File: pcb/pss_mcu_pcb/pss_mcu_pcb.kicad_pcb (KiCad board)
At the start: 4 copper layers, 30.1 x 47.4 mm, 50 parts, among them J1 STM32_Prog, J2 UART_Prog, J3 Conn_01x18, J4 Conn_01x18, SW1 Boot, SW2 EN, SW3 SW_Push, U1 LM3940IMP-3.3_NOPB, U2 LM358, U3 STM32F030K6Tx, U4 ESP32-WROOM-32U

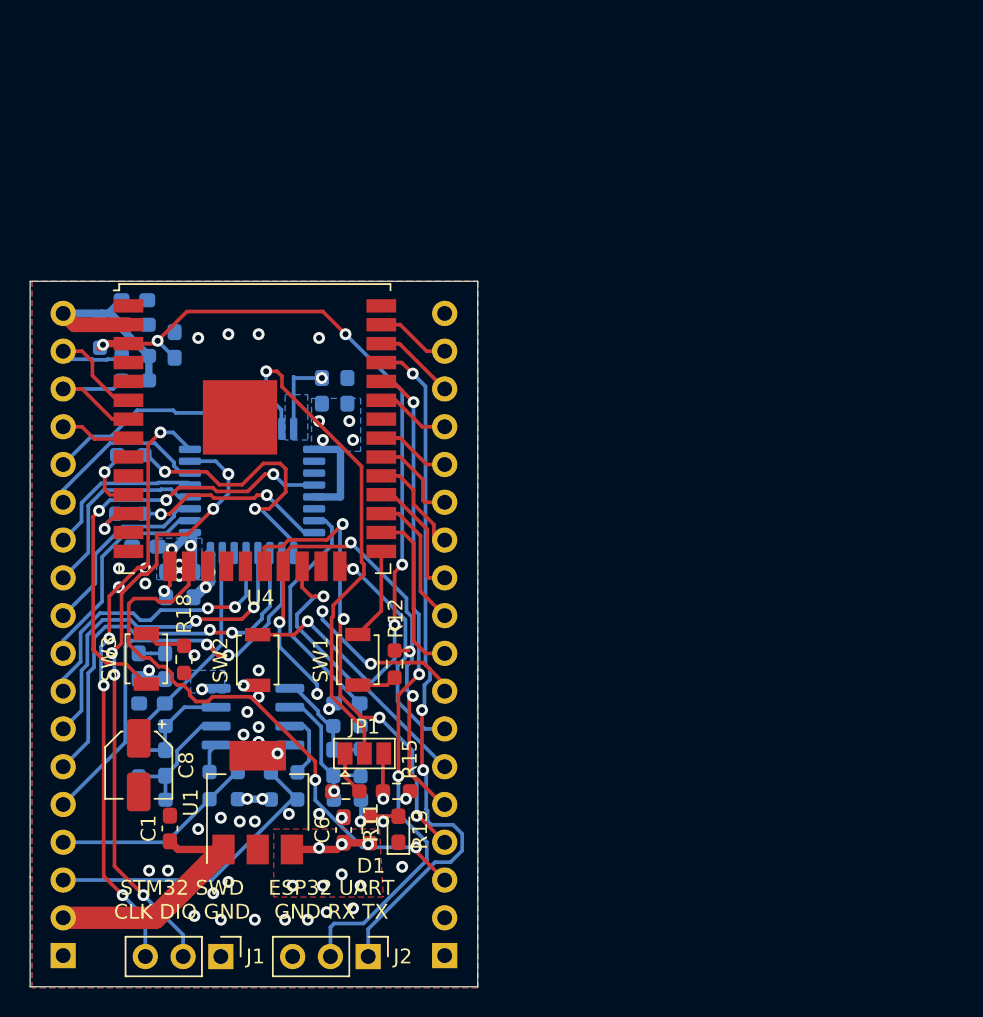
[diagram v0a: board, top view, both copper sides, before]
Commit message: Fix design issues
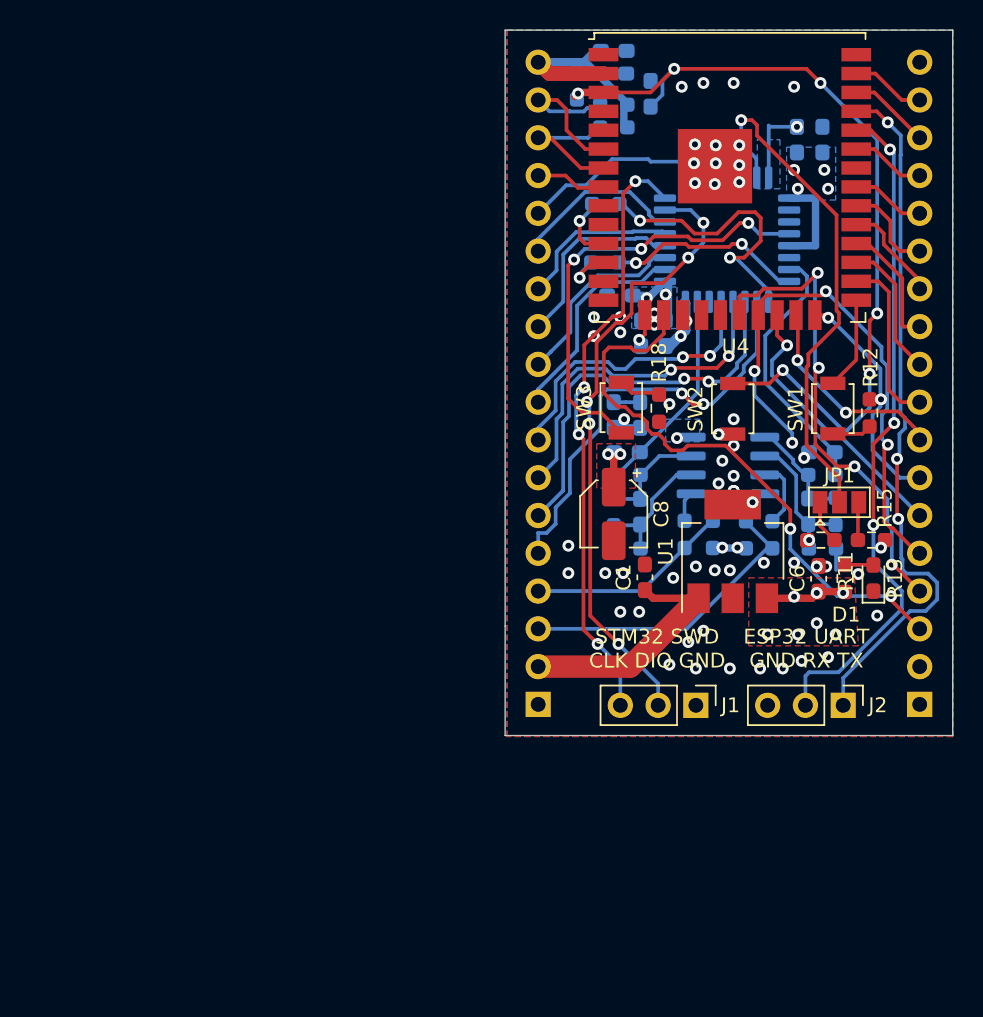
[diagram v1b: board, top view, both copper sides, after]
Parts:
- moved R16 36.4 mm to (150.4, 73.5)
- moved R14 36.3 mm to (150.4, 71.9)
- moved C5 36.3 mm to (150.3, 69.8)
- moved C3 36.3 mm to (150.4, 68.3)
- moved C17 36.2 mm to (152.8, 71.2)
- moved R17 36.2 mm to (147.9, 70.7)
- moved C1 36.1 mm to (152.5, 103.7)
- moved C10 36.1 mm to (163.4, 99.3)
- moved C2 36.1 mm to (162.7, 74.3)
- moved D1 36.1 mm to (167.8, 103.8)
- moved R11 36.1 mm to (164.3, 101.2)
- moved R12 36.1 mm to (167.6, 92.7)
- moved R2 36.1 mm to (157.0, 100.8)
- moved R5 36.1 mm to (155.1, 100.8)
- moved R7 36.1 mm to (165.3, 99.3)
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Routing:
- net DISP_T_DO: track 11.1 -> 14.1 mm
- net +3V3: track 44.2 -> 46.6 mm, vias 20 -> 22
- net SD_SDO: track 20.0 -> 18.6 mm
- net EN: track 55.5 -> 56.8 mm
- net GND: track 16.7 -> 16.5 mm, vias 49 -> 61
